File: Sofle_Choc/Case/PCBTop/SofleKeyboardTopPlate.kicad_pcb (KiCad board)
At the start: 2 copper layers, 143.4 x 111.8 mm, 34 parts, among them SW2 KEY_SWITCH

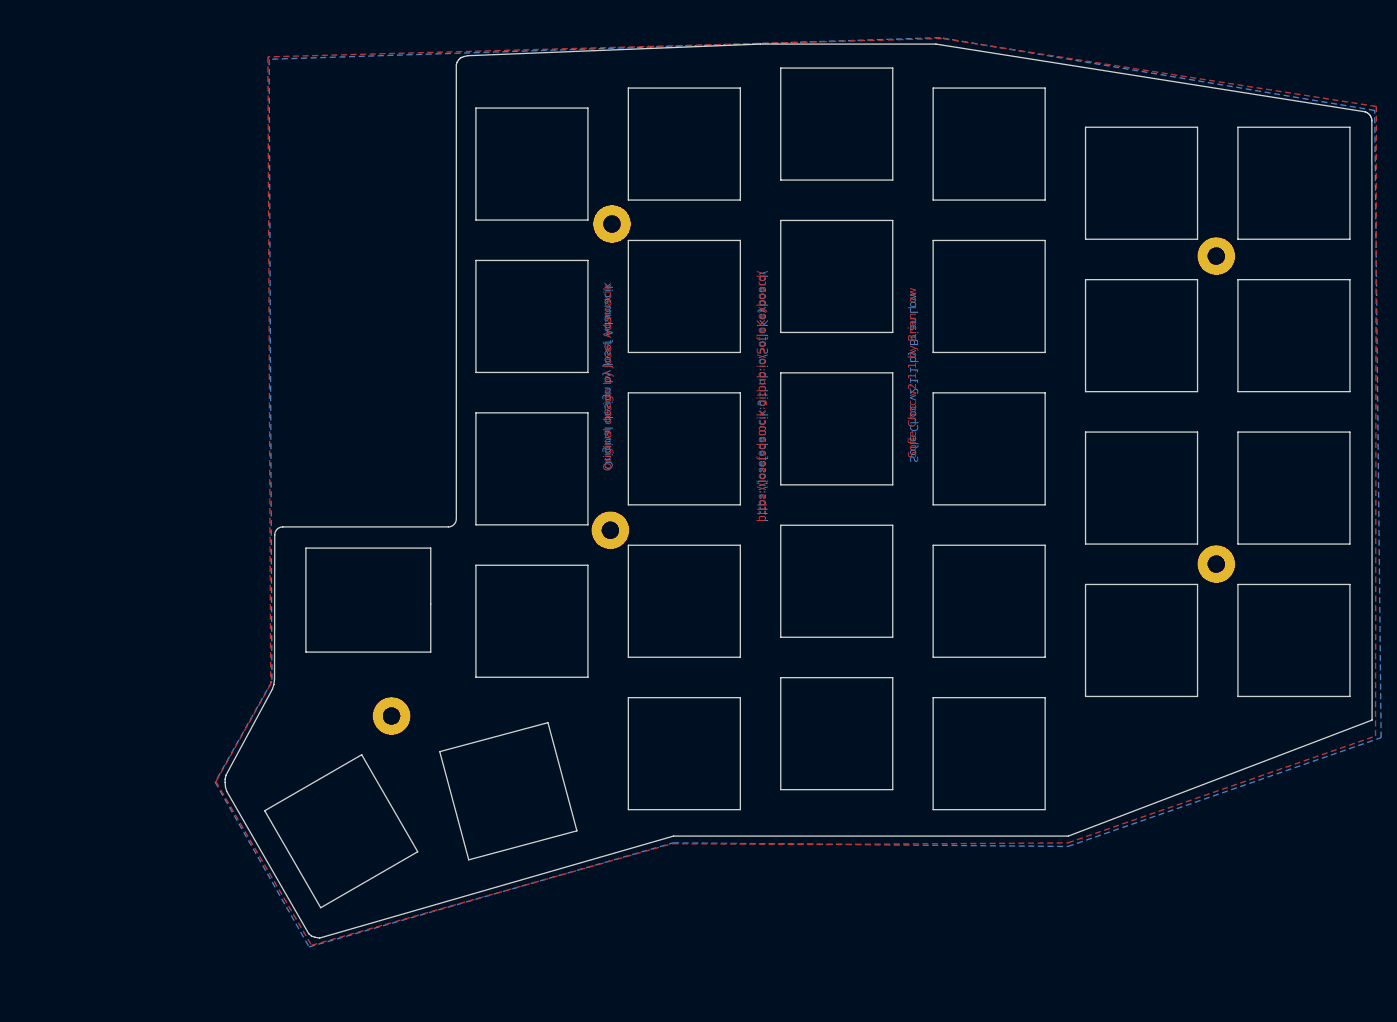
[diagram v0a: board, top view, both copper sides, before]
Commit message: Cleanup
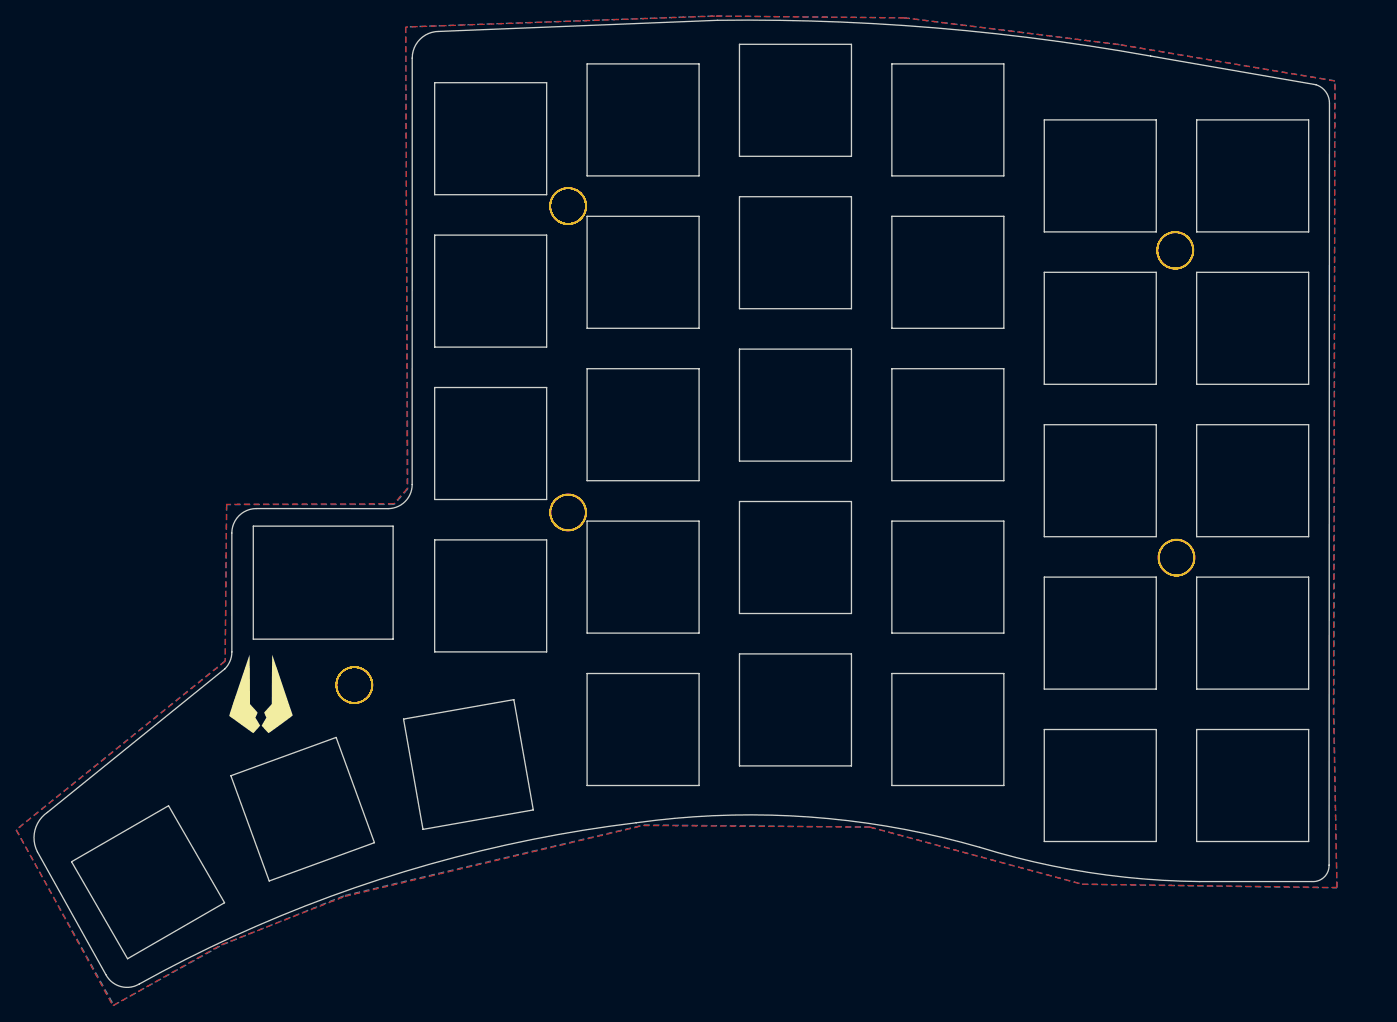
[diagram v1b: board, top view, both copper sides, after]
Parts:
- removed SW2 (x29): KEY_SWITCH, SofleChocTop:SW_Hole
- removed the TH3 at (131.4, 59.0)
- removed the TH4 at (207.2, 63.2)
- removed the TH7 at (103.9, 120.4)
- added ? (x2): , , F.Cu at (99.2, 116.6)
- added ? (x2): , , F.Cu at (126.0, 56.7)
- added ?: , , F.Cu at (126.0, 95.0)
- added ?: , , F.Cu at (201.9, 62.2)
- added ?: , , F.Cu at (202.0, 100.6)
- added ?: , , F.Cu at (201.9, 62.3)
- added G***: LOGO, LOGO, F.Cu at (87.6, 117.7)
- added G***: LOGO, LOGO, B.Cu at (87.6, 117.7)
- added TH3 (x2): HOLE, SofleKeyboard-footprint:HOLE_M2_TH, F.Cu at (125.9, 56.8)
- added TH4: HOLE, SofleKeyboard-footprint:HOLE_M2_TH, F.Cu at (202.1, 62.6)
- added TH4: HOLE, SofleKeyboard-footprint:HOLE_M2_TH, F.Cu at (202.1, 62.5)
- added TH7 (x2): HOLE, SofleKeyboard-footprint:HOLE_M2_TH, F.Cu at (99.2, 116.6)
- moved TH5 5.73 mm to (126.0, 95.1)
- moved TH6 5.04 mm to (202.2, 100.7)
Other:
- board size 143.4 x 111.8 mm -> 161.9 x 120.9 mm
- net class Default removed
- rule pad_to_mask_clearance: 0.2 -> 0
- board text removed: "Original design by Josef Adamacik"
- board text removed: "Sofle Choc v2.1.1 by Brian Low"
- board text removed: "https://josefadamcik.github.io/SofleKeyboard/"
